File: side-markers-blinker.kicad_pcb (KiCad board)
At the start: 2 copper layers, 130 x 100 mm, 35 parts, among them J1 Conn_01x04_Socket, J2 Conn_01x02_Socket, J3 Conn_01x04_Socket, J4 Conn_01x02_Socket, Q1 IRF540N, Q2 BC546, Q3 BC546, Q4 IRF540N, Q5 BC546, Q6 BC546

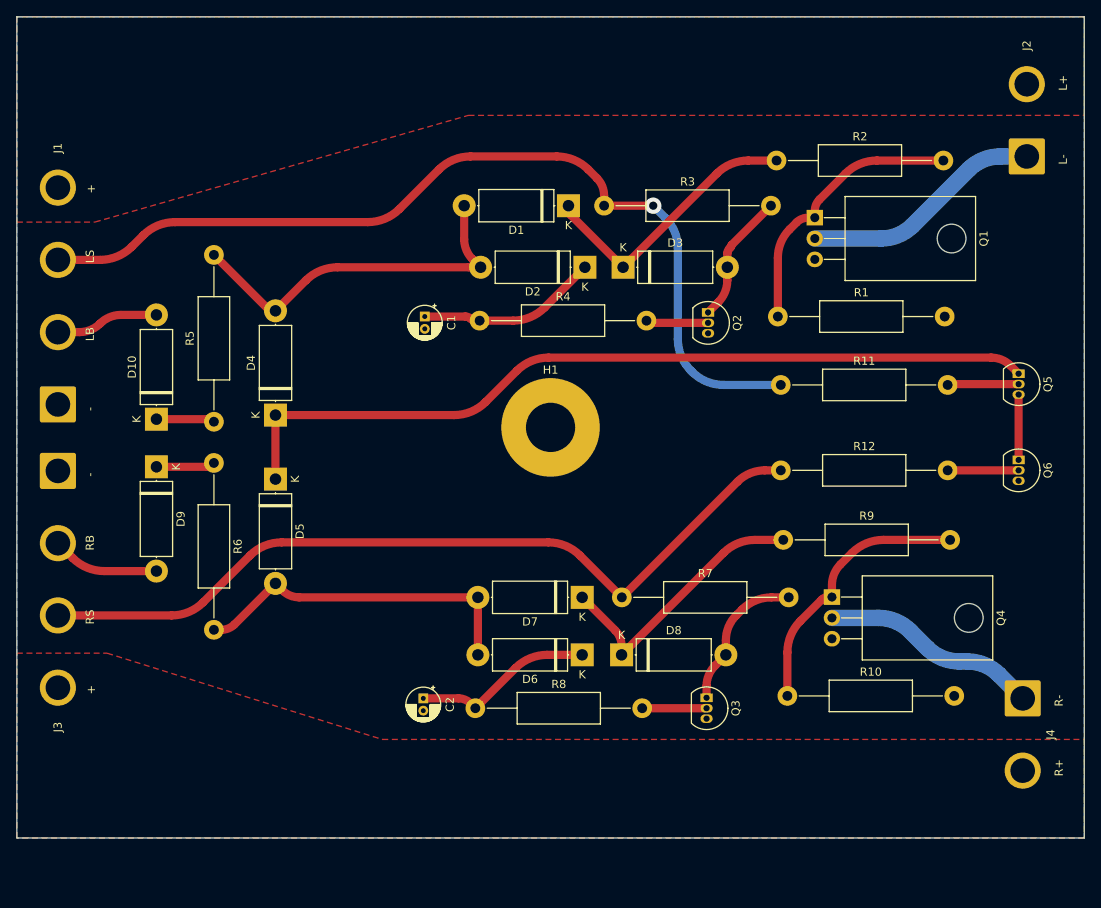
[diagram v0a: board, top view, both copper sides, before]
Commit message: Reduce board size.
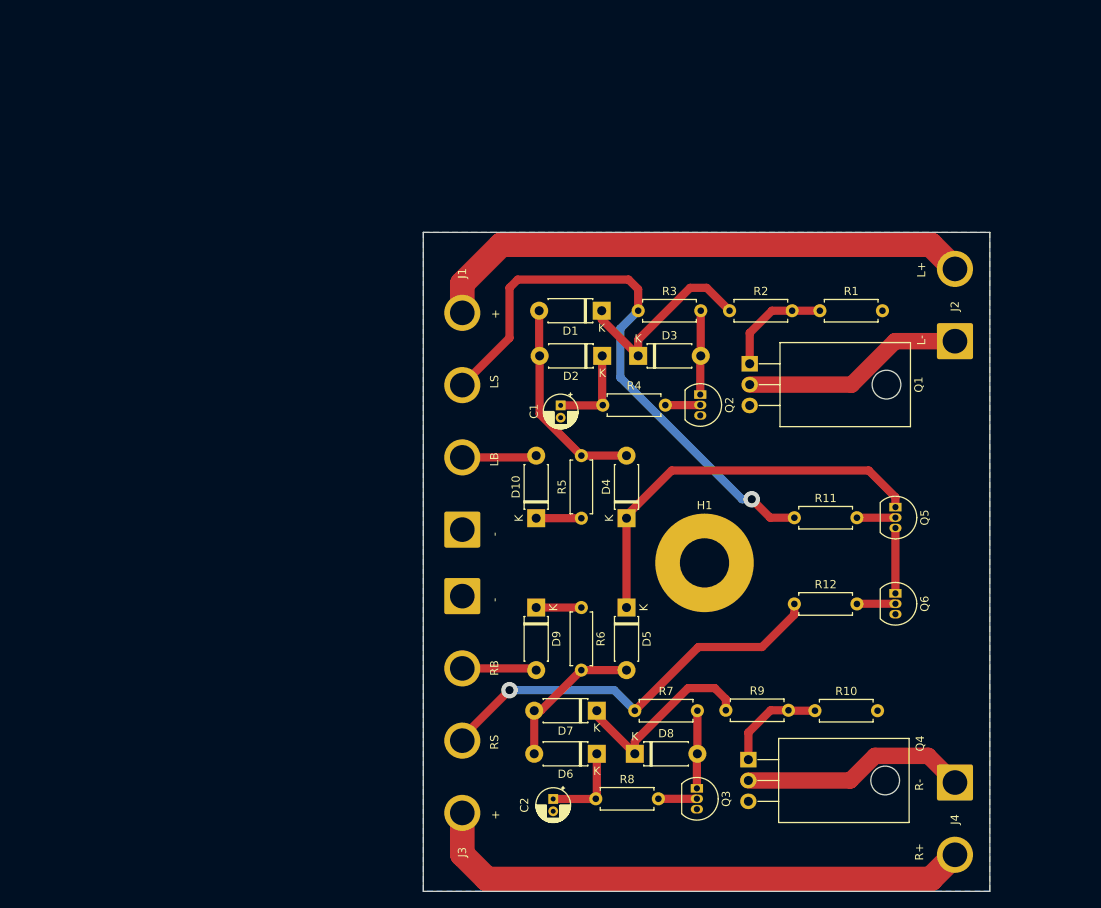
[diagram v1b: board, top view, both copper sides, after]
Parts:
- D1, D10, D2, D3, D4, D5, D6, D7, D8, D9: footprint Diode_THT:D_5W_P12.70mm_Horizontal -> Diode_THT:D_DO-41_SOD81_P7.62mm_Horizontal
- R1, R10, R11, R12, R2, R3, R4, R5, R6, R7, R8, R9: footprint Resistor_THT:R_Axial_DIN0411_L9.9mm_D3.6mm_P20.32mm_Horizontal -> Resistor_THT:R_Axial_DIN0207_L6.3mm_D2.5mm_P7.62mm_Horizontal
- moved J1 51.6 mm to (116.2, 95.0)
- moved J3 51.6 mm to (116.2, 103.0)
- moved D9 49.3 mm to (125.2, 104.4)
- moved R6 48.1 mm to (130.8, 104.4)
- moved D10 47.8 mm to (125.2, 93.6)
- moved R5 46.3 mm to (130.8, 93.6)
- moved D5 45.5 mm to (136.2, 104.4)
- moved D4 44.6 mm to (136.2, 93.6)
- moved H1 25.0 mm to (145.8, 99.0)
- moved J2 24.1 mm to (176.2, 72.0)
- moved Q4 22.3 mm to (151.1, 123.0)
- moved Q5 22.1 mm to (169.0, 92.2)
- moved Q6 22.1 mm to (169.0, 102.7)
- moved R9 21.9 mm to (148.3, 117.0)
- moved C2 20.0 mm to (127.3, 127.8)
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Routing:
- net Side marker lamp +24v R: track 0.00 -> 67.5 mm
- net Side marker lamp +24v L: track 0.00 -> 66.7 mm
- net AND gate: track 101.3 -> 48.8 mm
- net Side marker signal R: track 99.9 -> 50.4 mm, vias 0 -> 1
- net Side marker signal L: track 113.1 -> 70.7 mm
- net Net-(D5-A): track 41.7 -> 18.5 mm
- net Net-(Q4-G): track 32.9 -> 12.6 mm
- net Net-(Q1-G): track 33.3 -> 13.4 mm
- net Net-(D1-A): track 43.8 -> 25.3 mm
- net Net-(D6-K): track 21.8 -> 10.7 mm
- net Net-(D2-K): track 22.1 -> 11.2 mm
- net Net-(D1-K): track 34.0 -> 24.2 mm
- net Net-(D8-A): track 18.1 -> 9.48 mm
- net Net-(D7-K): track 32.9 -> 24.4 mm
- net Net-(D3-A): track 15.9 -> 10.2 mm
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- removed copper zone on F.Cu, net Side marker lamp +24v L
- removed copper zone on F.Cu, net Side marker lamp +24v R
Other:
- board size 130 x 100 mm -> 69 x 80.2 mm
